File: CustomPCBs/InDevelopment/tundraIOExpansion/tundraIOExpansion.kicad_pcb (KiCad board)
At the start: 4 copper layers, 46 x 36.5 mm, 83 parts, among them J1 Conn_01x25, T1 BSS138BKS_115, T2 BSS138BKS_115, T3 BSS138BKS_115, T4 BSS138BKS_115, T5 BSS138BKS_115, T6 BSS138BKS_115, T7 BSS138BKS_115, U1 RP2040, U2 RP2040, U3 MOUDLE-SEEEDUINO-XIAO-ESP32C3, U4 HE6206-18NR, U5 W25Q32JVSS, U6 W25Q32JVSS, Y1 12.000MHz, Y2 12.000MHz

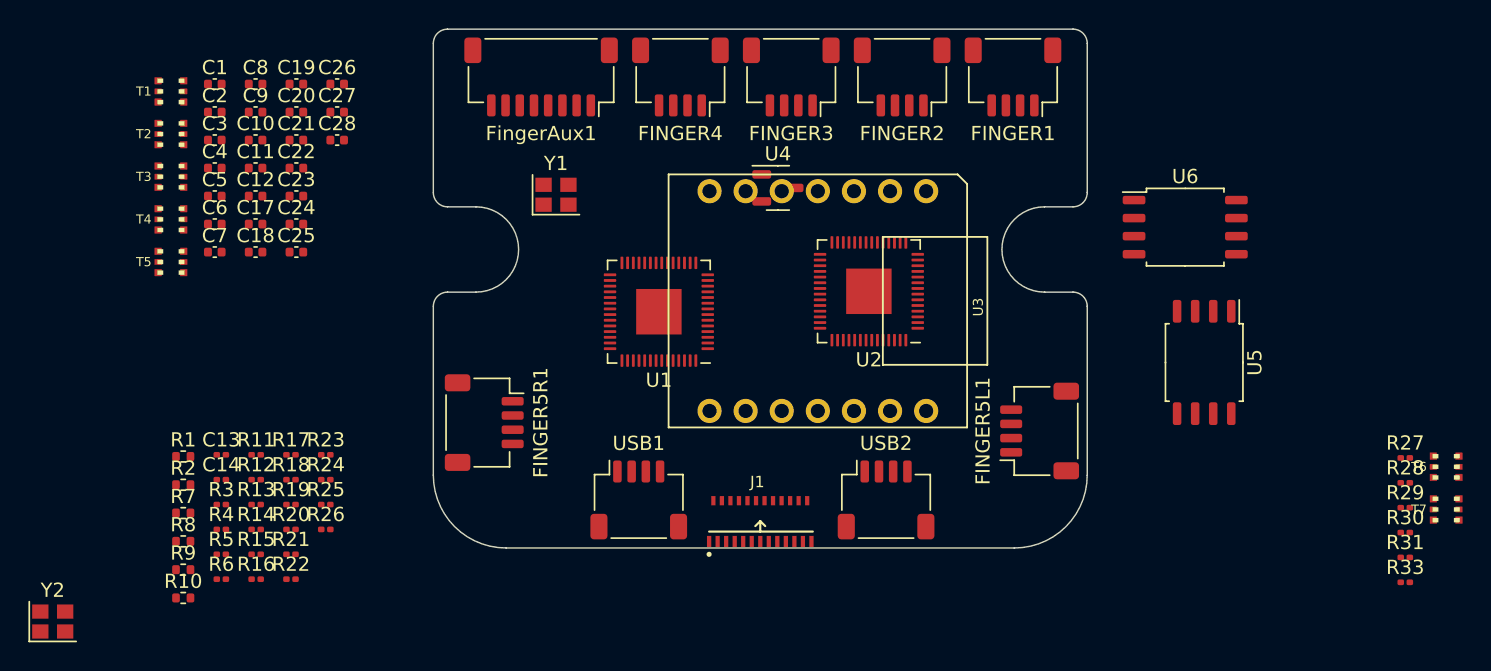
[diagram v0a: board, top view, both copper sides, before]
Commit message: Part positions more or less finished on main board
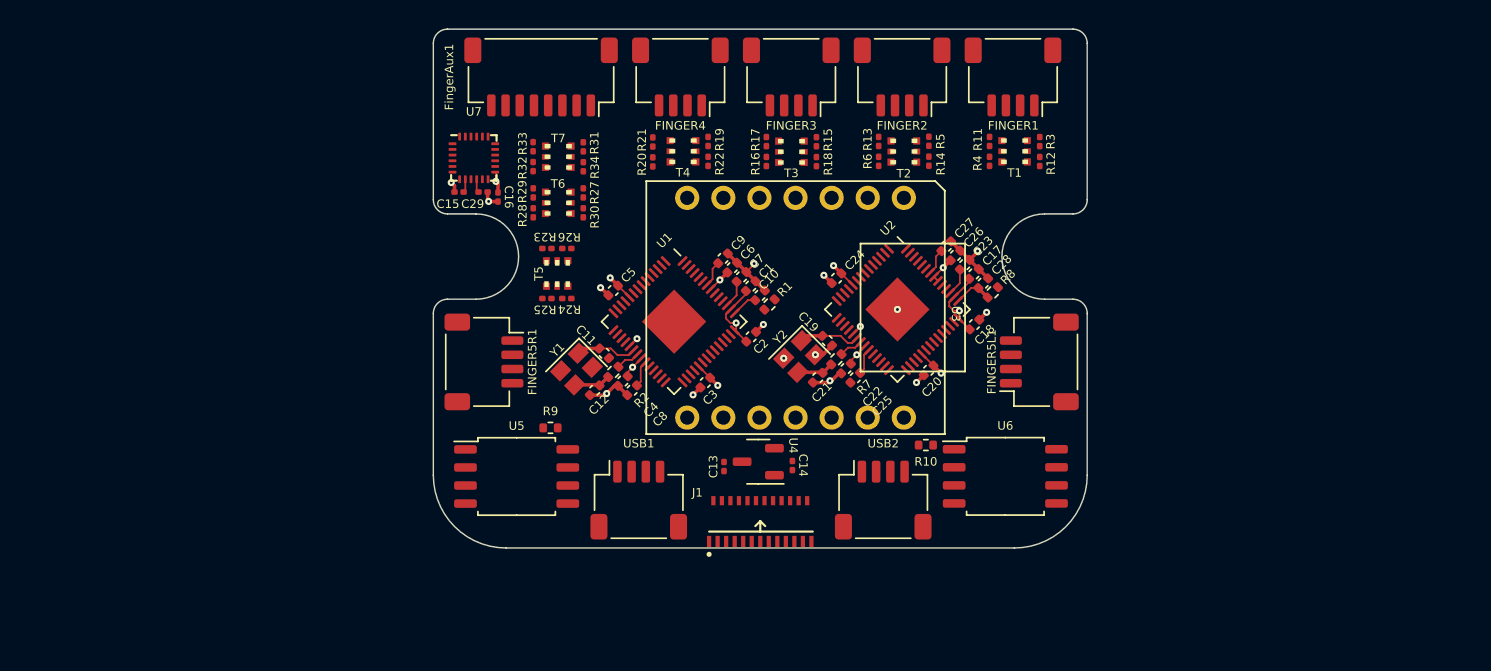
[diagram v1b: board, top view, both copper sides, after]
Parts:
- added C15: 100n, Capacitor_SMD:C_0201_0603Metric, F.Cu at (117.6, 68.0)
- added C16: 100n, Capacitor_SMD:C_0201_0603Metric, F.Cu at (120.3, 68.4)
- added C29: 100n, Capacitor_SMD:C_0201_0603Metric, F.Cu at (119.3, 68.0)
- added R32: 10k, Resistor_SMD:R_0201_0603Metric, F.Cu at (122.8, 66.3)
- added R34: 10k, Resistor_SMD:R_0201_0603Metric, F.Cu at (126.3, 66.3)
- added U7: ICM-20948, Sensor_Motion:InvenSense_QFN-24_3x3mm_P0.4mm, F.Cu at (118.6, 65.7)
- moved R33 68.6 mm to (122.8, 64.9), turned to 90 degrees
- moved T7 67.2 mm to (124.6, 65.6)
- moved R29 65.2 mm to (122.8, 68.1), turned to 90 degrees
- moved T6 65.2 mm to (124.6, 68.8)
- moved R31 64.6 mm to (126.3, 64.9), turned to -90 degrees
- moved R28 64.2 mm to (122.8, 69.5), turned to 90 degrees
- moved R3 63.0 mm to (158.4, 64.5), turned to -90 degrees
- moved R30 62.0 mm to (126.3, 69.5), turned to -90 degrees
- moved R27 60.8 mm to (126.3, 68.1), turned to -90 degrees
- moved R4 59.9 mm to (154.9, 65.9), turned to 90 degrees
- moved R8 59.6 mm to (155.1, 75.1), turned to -135 degrees
- moved T1 59.5 mm to (156.7, 65.2)
- moved R12 59.5 mm to (158.4, 65.9), turned to -90 degrees
- moved R5 57.6 mm to (150.6, 64.5), turned to -90 degrees
- moved R11 56.1 mm to (154.9, 64.5), turned to 90 degrees
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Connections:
- net SDI_1V8 renamed MISO_1V8
- net SDI_3V3 renamed MISO_3V3
- net SDO_1V8 renamed MOSI_1V8
- net SDO_3V3 renamed MOSI_3V3
- T7 pad 3: (no net) -> nCS_3V3
- T7 pad 4: (no net) -> nCS_1V8
- T7 pad 5: (no net) -> +1V8
- U3 pad 4: unconnected-(U3-PA11_A3_D3-Pad4) -> nCS_3V3
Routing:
- net +3V3: track 0.00 -> 24.8 mm, vias 0 -> 10
- net GND: track 0.00 -> 24.0 mm, vias 0 -> 17
- net Net-(U1-VREG_VOUT): track 0.00 -> 5.71 mm
- net Net-(U2-VREG_VOUT): track 0.00 -> 5.68 mm
- net Net-(U2-XIN): track 0.00 -> 4.40 mm
- net Net-(U1-XIN): track 0.00 -> 4.36 mm
- net Net-(U2-ADC_AVDD): track 0.00 -> 2.74 mm
- net Net-(C21-Pad1): track 0.00 -> 2.61 mm
- net Net-(C12-Pad1): track 0.00 -> 2.61 mm
- net +1V8: track 0.00 -> 2.46 mm, vias 0 -> 1
- net Net-(U1-ADC_AVDD): track 0.00 -> 1.81 mm
- net Net-(U2-XOUT): track 0.00 -> 1.72 mm
- net Net-(U1-XOUT): track 0.00 -> 1.71 mm
- net Net-(U7-REGOUT): track 0.00 -> 0.95 mm
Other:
- outline, holes or cut-outs redrawn
